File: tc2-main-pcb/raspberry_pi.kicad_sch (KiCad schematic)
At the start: 16 parts, among them J1 Screw_Terminal_01x01, J4 Raspberry_Pi_2_3, J5 Screw_Terminal_01x01, J6 Screw_Terminal_01x01, U13 MAX98357

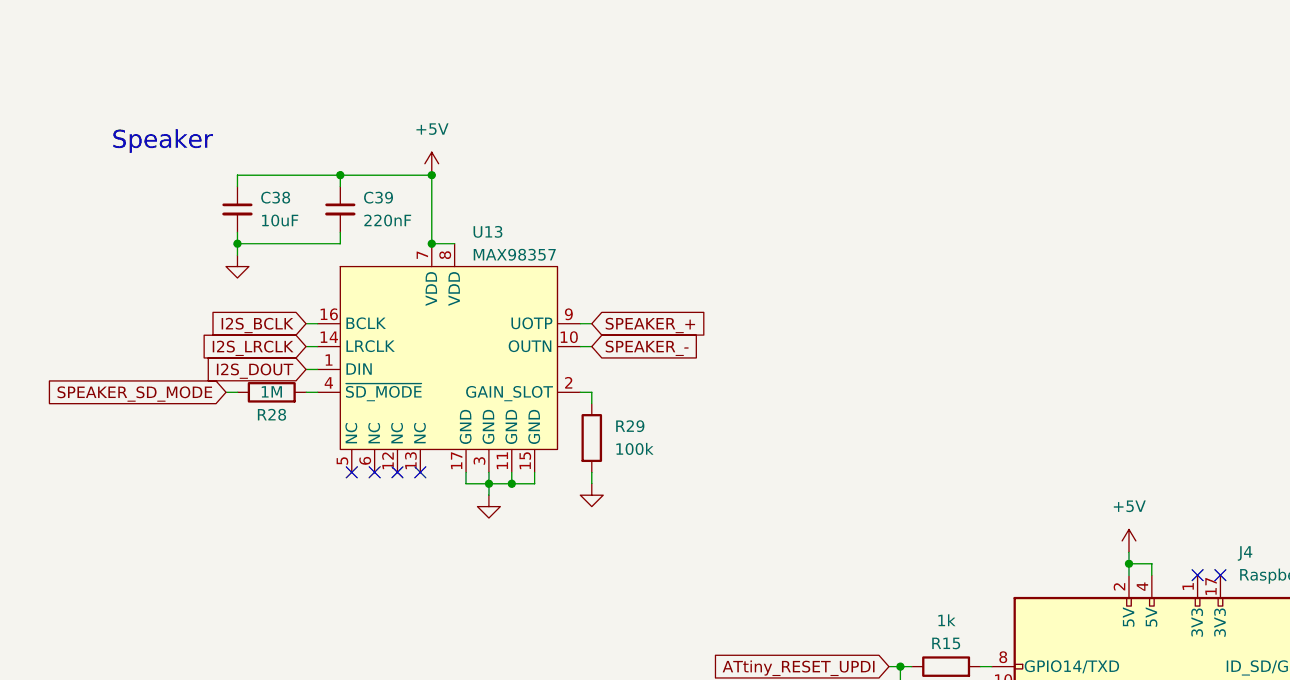
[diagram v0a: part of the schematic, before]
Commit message: Thermal camera V2 WIP
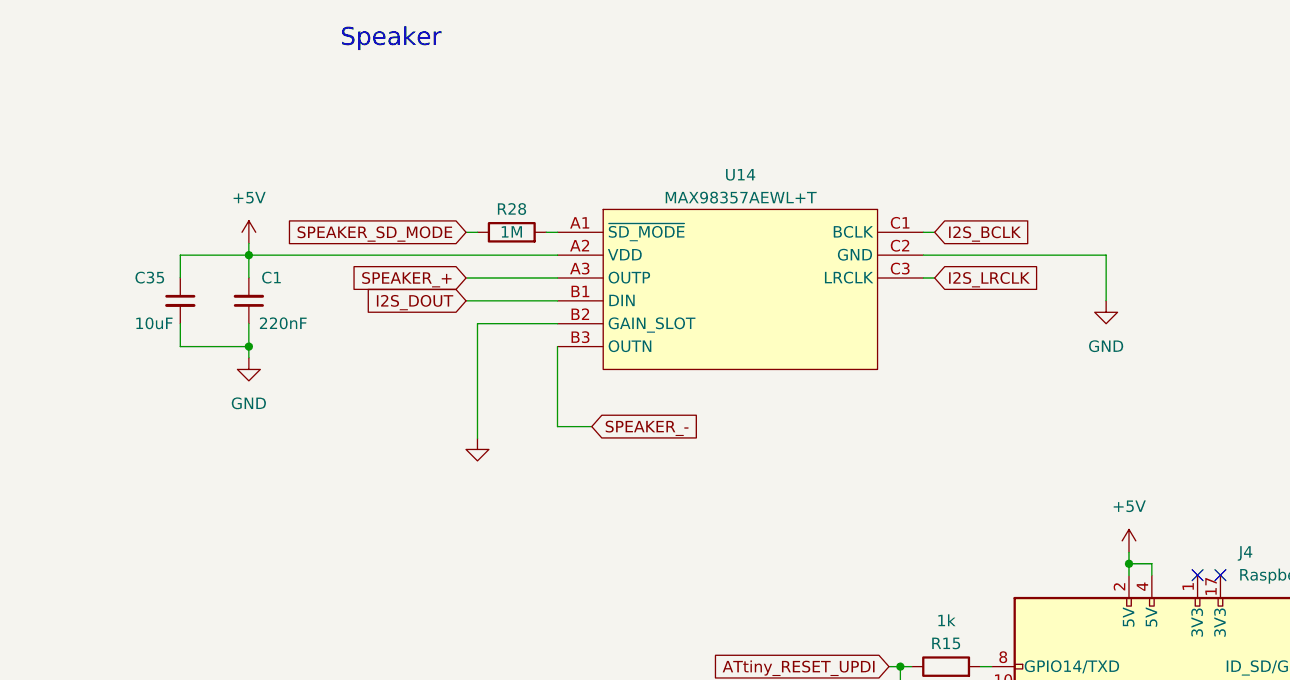
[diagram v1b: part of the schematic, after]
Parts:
- removed C38: 10uF, Capacitor_SMD:C_0603_1608Metric, symbol Device:C_Small
- removed C39: 220nF, Capacitor_SMD:C_0402_1005Metric, symbol Device:C_Small
- removed R29: 100k, Resistor_SMD:R_0402_1005Metric, symbol Device:R
- removed U13: MAX98357, Package_DFN_QFN:TQFN-16-1EP_3x3mm_P0.5mm_EP1.6x1.6mm, symbol cacophony-library:MAX98357
- added C1: 220nF, Capacitor_SMD:C_0402_1005Metric, symbol Device:C_Small
- added C35: 10uF, Capacitor_SMD:C_0603_1608Metric, symbol Device:C_Small
- added U14: MAX98357AEWL+T, cacophony-library:WLP-9_L1.4-W1.3-P0.40-R3-C3-BR, symbol cacophony-library:MAX98357AEWL+T
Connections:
- net +5V: now also C1.2, C35.1, U14.A2 (VDD)
- net GND: now also C1.1, C35.2, U14.B2 (GAIN_SLOT), U14.C2 (GND)
- net I2S_BCLK: now also U14.C1 (BCLK)
- net I2S_DOUT: now also U14.B1 (DIN)
- net I2S_LRCLK: now also U14.C3 (LRCLK)
- net SPEAKER_+: now also U14.A3 (OUTP)
- net SPEAKER_-: now also U14.B3 (OUTN)
- net at R28.2: now also U14.A1 (~{SD_MODE})
- no-connect marks 17 -> 13
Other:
- moved on the sheet: R28
